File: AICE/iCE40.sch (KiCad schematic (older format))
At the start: 75 parts, among them J1 Conn_02x10_Odd_Even, J2 Conn_02x10_Odd_Even, Q1 S8550, U1 ICE40UP5K-SG48ITR, U2 ASFLMB-24.00MHZ-LC-T, U3 SMS, U4 W25Q, U5 HX711

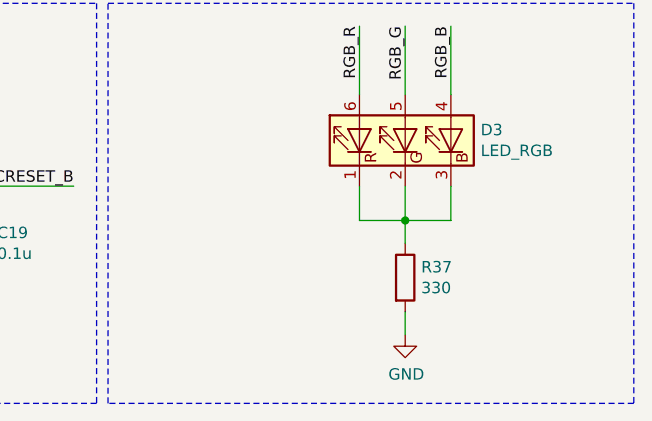
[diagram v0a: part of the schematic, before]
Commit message: Add files via upload
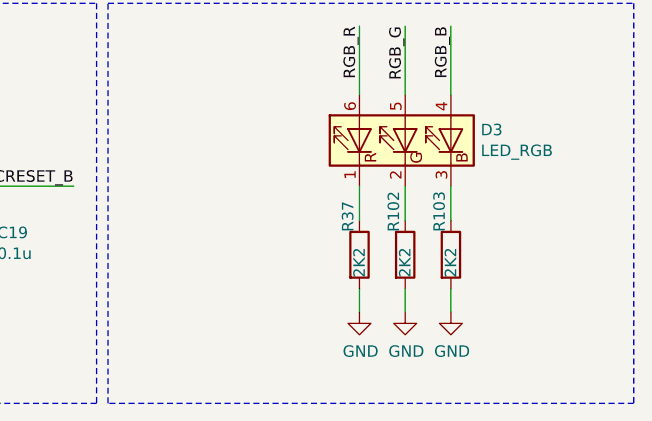
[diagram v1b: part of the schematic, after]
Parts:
- added R102, R103: 2K2, Resistor_SMD:R_0805_2012Metric_Pad1.15x1.40mm_HandSolder, symbol Device:R
- C1, C10, C11, C12, C13, C14, C15, C16, C17, C18, C19, C2, C5, C6, C7, C8: footprint (none) -> Capacitor_SMD:C_0805_2012Metric_Pad1.15x1.40mm_HandSolder
- C3, C4, C9: footprint (none) -> Capacitor_SMD:C_0603_1608Metric_Pad1.05x0.95mm_HandSolder
- D1, D2: footprint (none) -> LED_SMD:LED_0603_1608Metric_Pad1.05x0.95mm_HandSolder
- D3: footprint (none) -> LED_SMD:LED_RGB_Cree-PLCC-6_6x5mm_P2.1mm
- R1, R25, R26, R27, R3, R36, R4, R5, R6: footprint (none) -> Resistor_SMD:R_0603_1608Metric_Pad1.05x0.95mm_HandSolder
- R15, R16, R2: footprint (none) -> Resistor_SMD:R_0805_2012Metric_Pad1.15x1.40mm_HandSolder
- R37: value 330 -> 2K2; footprint (none) -> Resistor_SMD:R_0805_2012Metric_Pad1.15x1.40mm_HandSolder
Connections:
- net GND: now also R102.2, R103.2
- net at D3.1 (RK), R37.1: no longer D3.2 (GK), D3.3 (BK)
- new net: D3.2 (GK), R102.1
- new net: D3.3 (BK), R103.1
